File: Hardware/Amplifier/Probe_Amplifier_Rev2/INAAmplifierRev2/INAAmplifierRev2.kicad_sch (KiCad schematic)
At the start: 60 parts, among them J1 Conn_01x02, J10 Conn_01x01, J11 Conn_01x01, J12 Conn_01x04, J13 Conn_01x03, J14 Conn_01x04, J2 Conn_01x02, J3 Conn_01x02, J4 Conn_01x02, J5 Conn_01x02, J6 Conn_01x02, J7 Conn_01x02, J8 Conn_01x02, J9 Conn_01x02, U1 INA129, U2 LM358, U3 LM7805_TO220

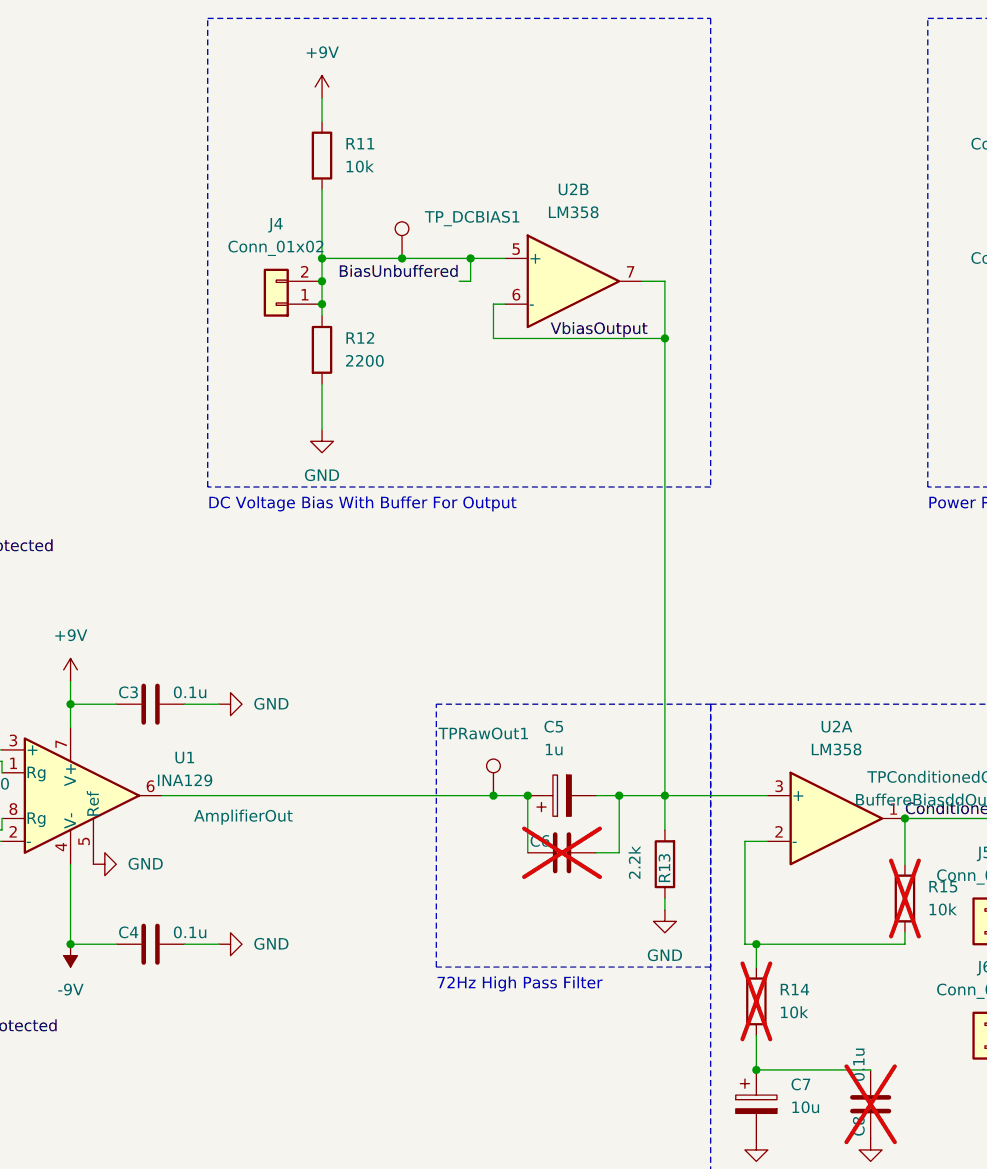
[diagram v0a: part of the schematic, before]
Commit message: fixed the INA AMplifer DC Bias Buffer
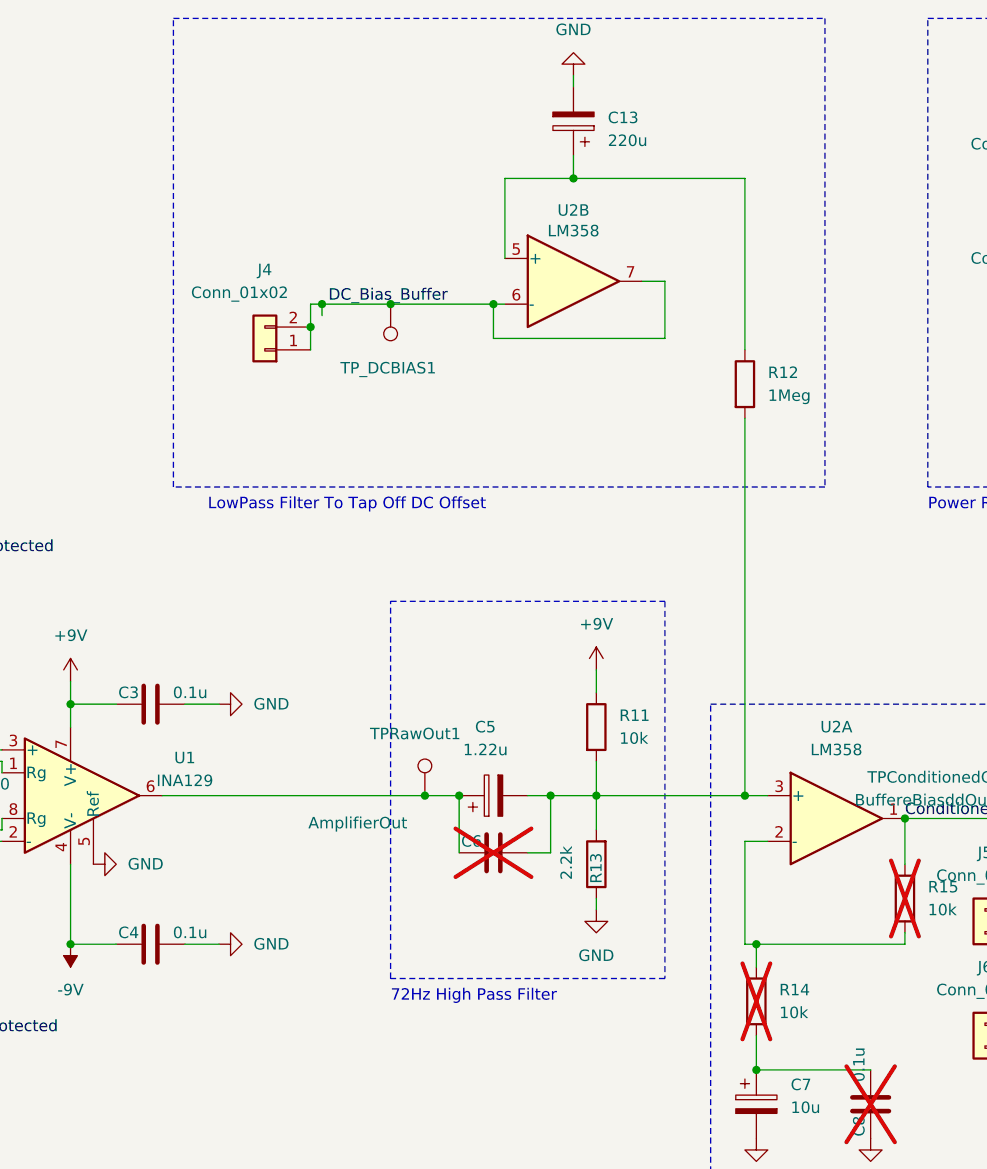
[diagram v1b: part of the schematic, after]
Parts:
- added C13: 220u, Capacitor_THT:CP_Radial_D6.3mm_P2.50mm, symbol Device:C_Polarized
- C5: value 1u -> 1.22u
- R12: value 2200 -> 1Meg
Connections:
- net GND: now also C13.2; no longer R12.2
- net BiasUnbuffered renamed DC_Bias_Buffer
- net DC_Bias_Buffer: now also U2.6 (-), U2.7; no longer R11.2, R12.1, U2.5 (+)
- net VbiasOutput: no longer names the net of C5.2, C6.2, R13.2, U2.3 (+)
- net VbiasOutput: now also R11.2, R12.2; no longer U2.6 (-), U2.7
- new net: C13.1, R12.1, U2.5 (+)
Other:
- note added: "LowPass Filter To Tap Off DC Offset"
- note removed: "DC Voltage Bias With Buffer For Output"
- moved on the sheet: C5, C6, R13, TPRawOut1
